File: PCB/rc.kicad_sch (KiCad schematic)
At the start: 24 parts, among them J1 Conn_01x03_Pin, J10 Conn_01x03_Pin, J11 Conn_01x03_Pin, J12 USB4120-03-C_REVA, J2 Conn_01x03_Pin, J3 Conn_01x03_Pin, J4 Conn_01x03_Pin, J5 Conn_01x03_Pin, J6 Conn_01x03_Pin, J7 Conn_01x03_Pin, J8 Conn_01x03_Pin, J9 Conn_01x03_Pin, SW1 SW_Push, U1 ME6211C33M5, U2 ESP32-S3-MINI-1U, U3 ESP32-C6-MINI-1/U

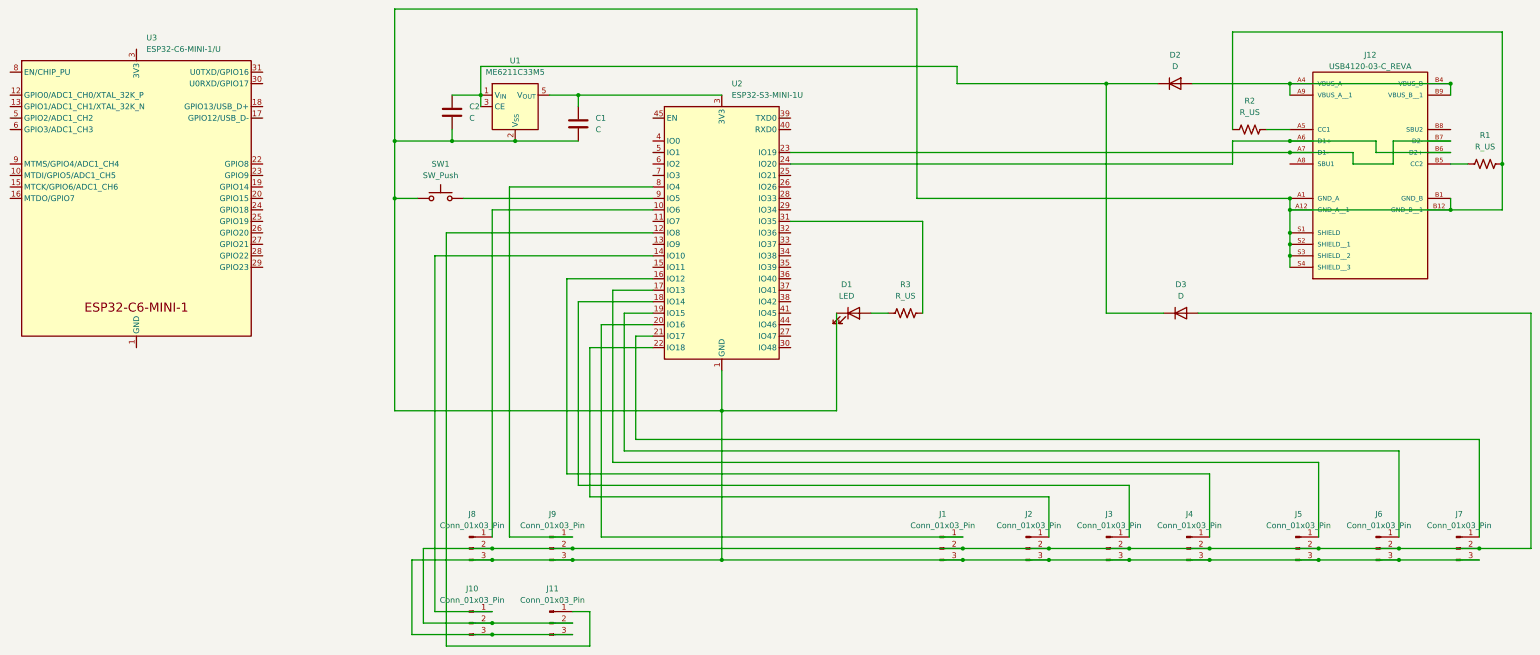
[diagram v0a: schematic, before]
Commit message: c6
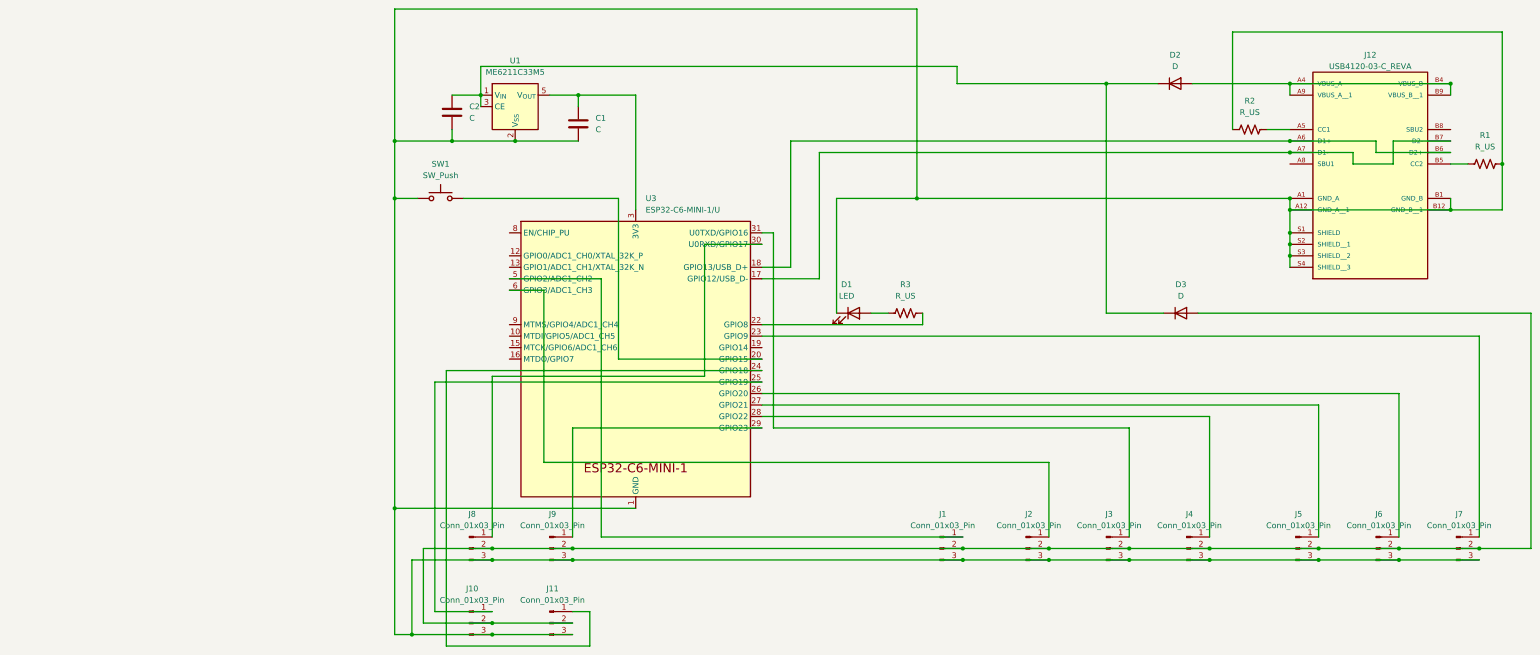
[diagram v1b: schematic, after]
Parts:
- removed U2: ESP32-S3-MINI-1U, RF_Module:ESP32-S2-MINI-1U, symbol RF_Module:ESP32-S3-MINI-1U
- D2, D3: footprint Diode_SMD:D_2010_5025Metric_Pad1.52x2.65mm_HandSolder -> Diode_SMD:D_0603_1608Metric_Pad1.05x0.95mm_HandSolder
- U3: footprint PCM_Espressif:ESP32-C6-MINI-1 -> PCM_Espressif:ESP32-C3-MINI-1_HandSoldering
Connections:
- net at U3.1 (GND), U3.11 (GND), U3.14 (GND)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: now also C1.2, C2.2, D1.1 (K), J1.3 (Pin_3), J10.3 (Pin_3), J11.3 (Pin_3), J12.A1 (GND_A), J12.A12 (GND_A__1), J12.B1 (GND_B), J12.B12 (GND_B__1), J12.S1 (SHIELD), J12.S2 (SHIELD__1), J12.S3 (SHIELD__2), J12.S4 (SHIELD__3), J2.3 (Pin_3), J3.3 (Pin_3), J4.3 (Pin_3), J5.3 (Pin_3), J6.3 (Pin_3), J7.3 (Pin_3), J8.3 (Pin_3), J9.3 (Pin_3), R1.1, R2.1, SW1.1, U1.2 (V_{SS})
- net at U3.17 (GPIO12/USB_D-): now also J12.A7 (D1-), J12.B7 (D2-)
- net at U3.18 (GPIO13/USB_D+): now also J12.A6 (D1+), J12.B6 (D2+)
- net at U3.20 (GPIO15): now also SW1.2
- net at U3.22 (GPIO8): now also R3.2
- net at U3.23 (GPIO9): now also J7.1 (Pin_1)
- net at U3.24 (GPIO18): now also J11.1 (Pin_1)
- net at U3.25 (GPIO19): now also J10.1 (Pin_1)
- net at U3.26 (GPIO20): now also J6.1 (Pin_1)
- net at U3.27 (GPIO21): now also J5.1 (Pin_1)
- net at U3.28 (GPIO22): now also J4.1 (Pin_1)
- net at U3.29 (GPIO23): now also J9.1 (Pin_1)
- net at U3.3 (3V3): now also C1.1, U1.5 (V_{OUT})
- net at U3.30 (U0RXD/GPIO17): now also J8.1 (Pin_1)
- net at U3.31 (U0TXD/GPIO16): now also J3.1 (Pin_1)
- net at U3.5 (GPIO2/ADC1_CH2): now also J1.1 (Pin_1)
- net at U3.6 (GPIO3/ADC1_CH3): now also J2.1 (Pin_1)
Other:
- moved on the sheet: U3
